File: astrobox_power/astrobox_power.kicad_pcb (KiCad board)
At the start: 2 copper layers, 122 x 105 mm, 61 parts, among them J10 FAN_AUTO, J6 INTERCOM1, J7 POWER_OUT, J8 PWR_IN, J9 PWR_IN_BAT, K1 G5LE-1, K2 G5LE-1, K3 G5LE-1, K4 G5LE-1, Q1 IRF4905, Q2 BUZ11, Q3 IRLZ34N, Q4 IRLZ34N, SW5 SW_PWR_ON, U1 MC34063AP, U2 L7812, U3 L7805, U4 ATtiny85-20P, U5 DHT11, U6 4N25

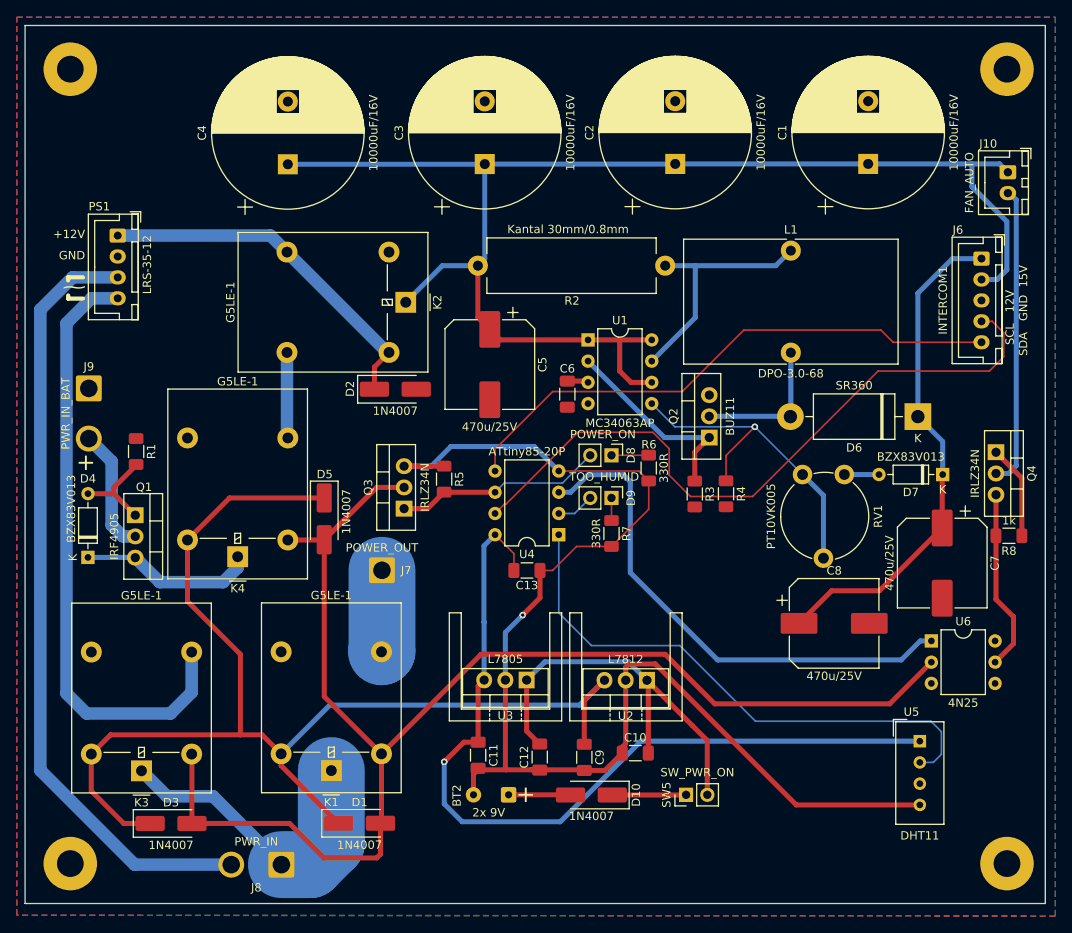
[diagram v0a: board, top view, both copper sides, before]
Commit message: astrobox WIP
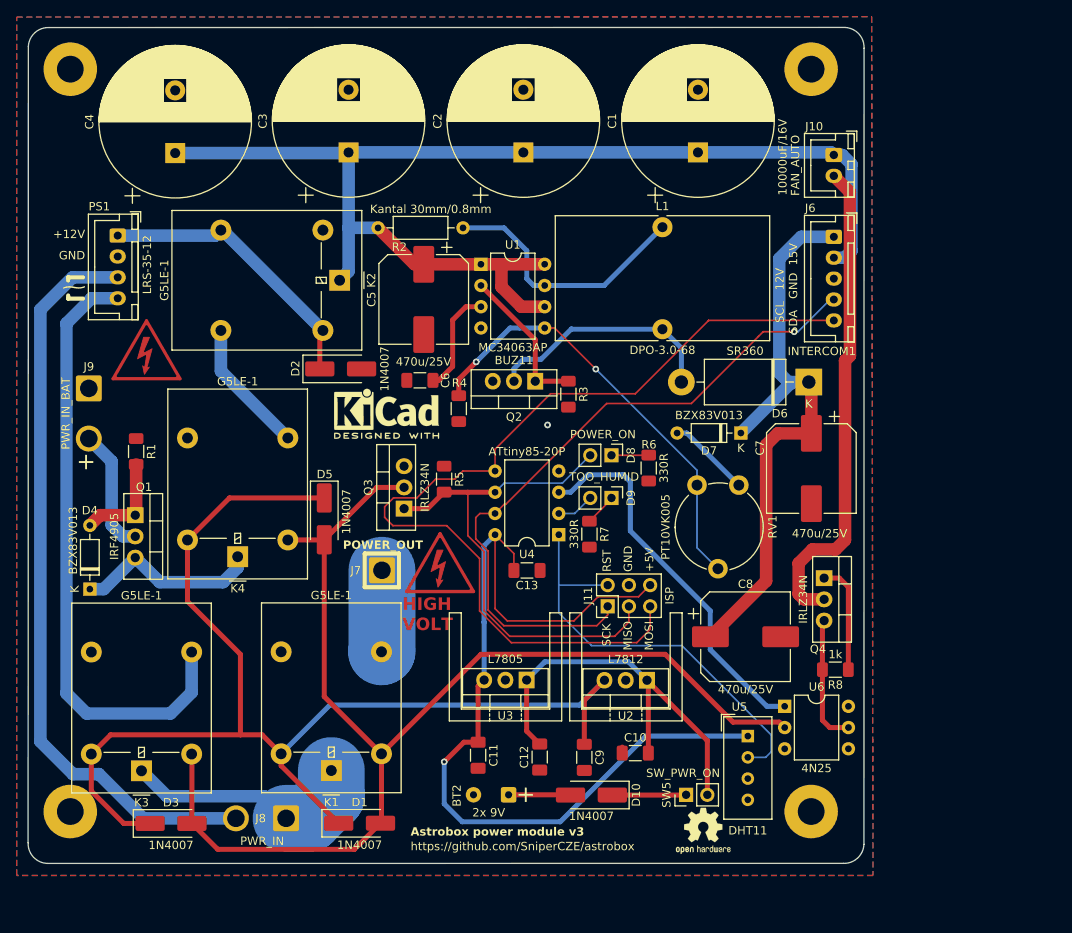
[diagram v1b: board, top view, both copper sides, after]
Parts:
- added J11: ISP, Connector_PinHeader_2.54mm:PinHeader_2x03_P2.54mm_Vertical, F.Cu at (137.7, 110.5)
- added REF**: Symbol_HighVoltage_Triangle_8x7mm_Copper, Symbol:Symbol_HighVoltage_Triangle_8x7mm_Copper, F.Cu at (82.5, 79.8)
- added REF**: OSHW-Logo2_7.3x6mm_SilkScreen, Symbol:OSHW-Logo2_7.3x6mm_SilkScreen, F.Cu at (149.1, 137.3)
- added REF**: Symbol_HighVoltage_Triangle_8x7mm_Copper, Symbol:Symbol_HighVoltage_Triangle_8x7mm_Copper, F.Cu at (117.6, 105.2)
- added REF**: KiCad-Logo2_5mm_SilkScreen, Symbol:KiCad-Logo2_5mm_SilkScreen, F.Cu at (111.2, 87.4)
- R2: footprint Resistor_THT:R_Axial_Power_L20.0mm_W6.4mm_P22.40mm -> Resistor_THT:R_Axial_DIN0207_L6.3mm_D2.5mm_P10.16mm_Horizontal
- moved R4 33.5 mm to (119.9, 86.8)
- moved R8 26.2 mm to (164.9, 118.0)
- moved Q4 25.5 mm to (163.6, 107.1)
- moved D7 24.6 mm to (153.6, 89.7)
- moved REF** 24.2 mm to (162.0, 135.0)
- moved REF** 23.4 mm to (162.0, 46.2)
- moved Q2 21.9 mm to (129.0, 83.5), turned to 180 degrees
- moved J10 20.9 mm to (164.7, 56.5)
- moved U5 20.6 mm to (154.4, 126.0)
- moved C1 20.4 mm to (148.5, 56.2)
- moved C7 19.3 mm to (162.0, 94.0)
- moved R3 19.3 mm to (133.0, 85.1)
- moved U6 19.2 mm to (158.8, 122.4)
- moved C2 18.2 mm to (127.6, 56.2)
- moved J6 17.9 mm to (164.7, 66.3)
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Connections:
- BT2 pad 2: Net-(BT2--) -> GND
- C10 pad 1: Net-(BT2--) -> GND
- C11 pad 2: Net-(BT2--) -> GND
- C12 pad 1: Net-(BT2--) -> GND
- C13 pad 2: Net-(BT2--) -> GND
- C9 pad 2: Net-(BT2--) -> GND
- Q3 pad 3: Net-(BT2--) -> GND
- R5 pad 1: Net-(BT2--) -> GND
- R6 pad 1: Net-(BT2--) -> GND
- R7 pad 2: Net-(BT2--) -> GND
- U2 pad 2: Net-(BT2--) -> GND
- U3 pad 2: Net-(BT2--) -> GND
- U4 pad 4: Net-(BT2--) -> GND
- U5 pad 4: Net-(BT2--) -> GND
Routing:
- net Net-(BT2--): track 156.0 -> 0.00 mm, vias 1 -> 0
- net /Internal_Bat_Subsystem/SDA: track 67.3 -> 110.8 mm
- net Net-(D8-A): track 24.9 -> 61.1 mm
- net Net-(J10-Pin_2): track 35.9 -> 58.3 mm
- net /Internal_Bat_Subsystem/INTBAT_GND: track 164.7 -> 143.2 mm
- net +12V: track 163.6 -> 144.1 mm
- net /Internal_Bat_Subsystem/PWM_FAN: track 61.9 -> 45.5 mm
- net Net-(J11-Pin_2): track 66.7 -> 51.7 mm
- net Net-(U1-Vfb): track 40.5 -> 52.8 mm, vias 1 -> 2
- net /StepUp_15V/15V: track 60.5 -> 71.7 mm
- net Net-(D6-A): track 17.4 -> 28.5 mm
- net Net-(U1-TC): track 2.54 -> 12.6 mm
- net Net-(J11-Pin_6): track 102.7 -> 112.1 mm
- net Net-(D2-K): track 43.4 -> 34.5 mm
- net Net-(J8-Pin_1): track 37.1 -> 29.2 mm
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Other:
- board size 122 x 105 mm -> 100 x 100 mm
- board text added: "+5V"
- board text added: "Astrobox power module v3"
- board text added: "HIGH VOLT"
- board text added: "MISO"
- board text added: "MOSI"
- board text added: "RST"
- board text added: "SCK"
- board text added: "https://github.com/SniperCZE/astrobox"
